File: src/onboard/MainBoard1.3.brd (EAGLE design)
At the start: 134.6 x 80.5 mm, 73 parts, among them IC1 MIC29310-5.0BT, IC2 ADAFRUIT_BMP280, IC3 A5975D

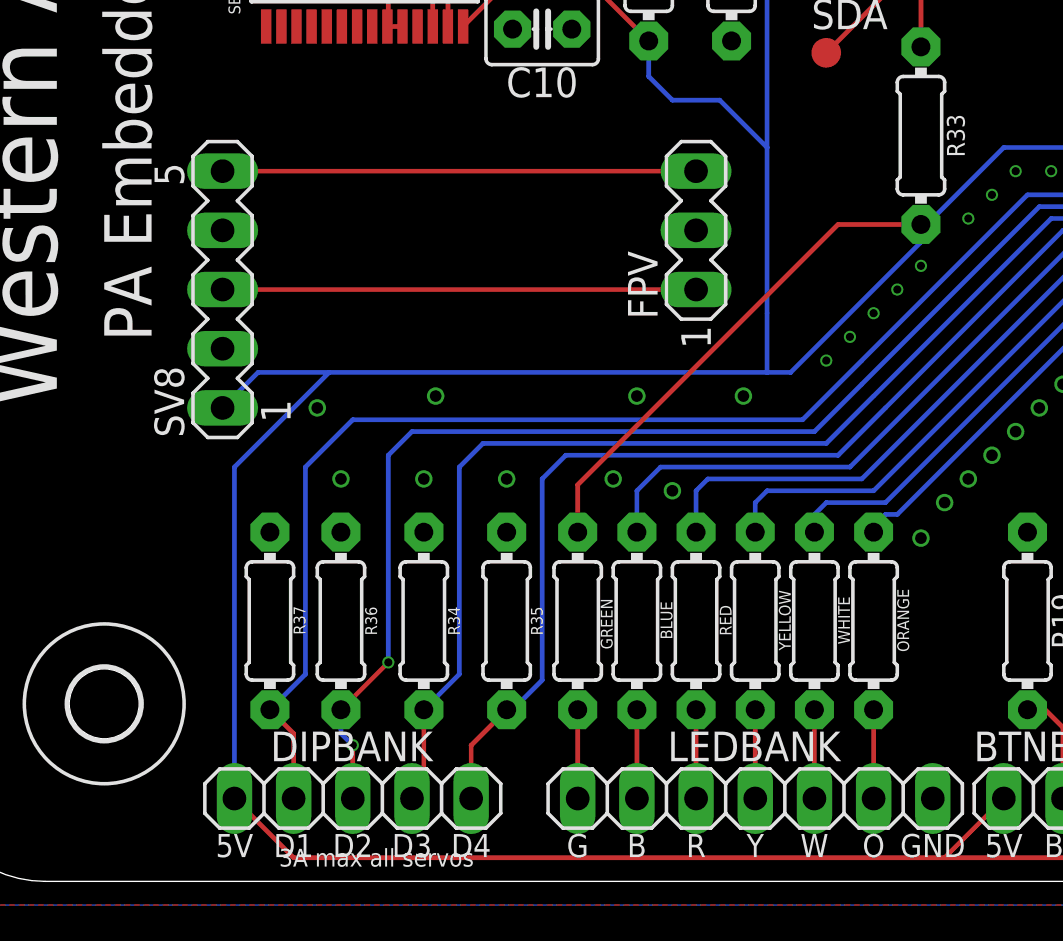
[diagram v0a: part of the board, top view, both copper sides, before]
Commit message: AKK iteration (incomplete)
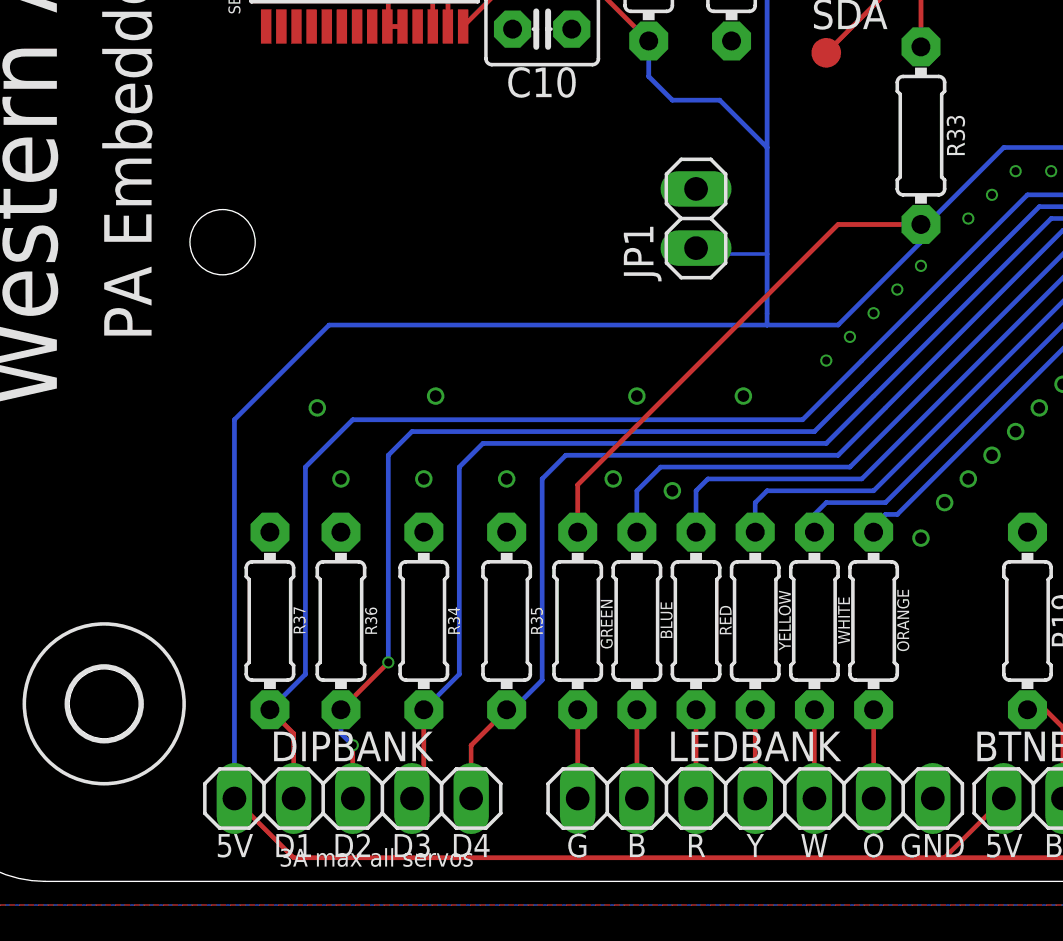
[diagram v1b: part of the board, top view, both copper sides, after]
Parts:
- removed FPV: (no value), con-lstb:MA03-1
- removed SV8: (no value), con-lstb:MA05-1
- added JP1: (no value), pinhead:1X02
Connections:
- removed net VIDEO: FPV.3, SV8.5
- net 5V: now also JP1.1; no longer FPV.1, SV8.1, SV8.3
- net GND: now also JP1.2; no longer FPV.2, SV8.2, SV8.4
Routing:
- net 5V: track 529.3 -> 506.1 mm
- net VIDEO: track 20.3 -> 0.00 mm
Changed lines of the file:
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@@
 <text x="133.096" y="40.259" size="1.778" layer="26" rot="MR90" align="center">Well...it can't get much worse</text>
 <text x="110.236" y="2.159" size="1.778" layer="26" rot="MR180" align="center">It's time to buzz the tower</text>
+<hole x="12.7" y="27.432" drill="2.8"/>
 </plain>
 <attributes>
@@
 <attribute name="VALUE" x="59.69" y="44.704" size="1.27" layer="27" rot="R90" align="center"/>
 </element>
-<element name="FPV" library="con-lstb" library_urn="urn:adsk.eagle:library:162" package="MA03-1" package3d_urn="urn:adsk.eagle:package:8339/1" value="" x="33.02" y="27.94" smashed="yes" rot="R90">
-<attribute name="MF" value="" x="33.02" y="27.94" size="1.778" layer="27" rot="R90" display="off"/>
-<attribute name="MPN" value="" x="33.02" y="27.94" size="1.778" layer="27" rot="R90" display="off"/>
-<attribute name="NAME" x="31.369" y="24.13" size="1.27" layer="25" ratio="10" rot="R90"/>
-<attribute name="OC_FARNELL" value="unknown" x="33.02" y="27.94" size="1.778" layer="27" rot="R90" display="off"/>
-<attribute name="OC_NEWARK" value="unknown" x="33.02" y="27.94" size="1.778" layer="27" rot="R90" display="off"/>
-<attribute name="POPULARITY" value="48" x="33.02" y="27.94" size="1.778" layer="27" rot="R90" display="off"/>
-<attribute name="VALUE" x="35.941" y="24.13" size="1.27" layer="27" ratio="10" rot="R90"/>
-</element>
-<element name="SV8" library="con-lstb" library_urn="urn:adsk.eagle:library:162" package="MA05-1" package3d_urn="urn:adsk.eagle:package:8332/1" value="" x="12.7" y="25.4" smashed="yes" rot="R90">
-<attribute name="MF" value="" x="12.7" y="25.4" size="1.778" layer="27" rot="R90" display="off"/>
-<attribute name="MPN" value="" x="12.7" y="25.4" size="1.778" layer="27" rot="R90" display="off"/>
-<attribute name="NAME" x="11.049" y="19.05" size="1.27" layer="25" ratio="10" rot="R90"/>
-<attribute name="OC_FARNELL" value="unknown" x="12.7" y="25.4" size="1.778" layer="27" rot="R90" display="off"/>
-<attribute name="OC_NEWARK" value="unknown" x="12.7" y="25.4" size="1.778" layer="27" rot="R90" display="off"/>
-<attribute name="POPULARITY" value="29" x="12.7" y="25.4" size="1.778" layer="27" rot="R90" display="off"/>
-<attribute name="VALUE" x="15.621" y="22.86" size="1.27" layer="27" ratio="10" rot="R90"/>
+<element name="JP1" library="pinhead" library_urn="urn:adsk.eagle:library:325" package="1X02" package3d_urn="urn:adsk.eagle:package:22435/2" value="" x="33.02" y="28.448" smashed="yes" rot="R90">
+<attribute name="NAME" x="31.1912" y="25.8318" size="1.27" layer="25" ratio="10" rot="R90"/>
+<attribute name="POPULARITY" value="98" x="33.02" y="28.448" size="1.778" layer="27" rot="R90" display="off"/>
+<attribute name="VALUE" x="36.195" y="25.908" size="1.27" layer="27" rot="R90"/>
 </element>
 </elements>
@@
 <wire x1="32.004" y1="33.528" x2="30.988" y2="34.544" width="0.2032" layer="16"/>
 <wire x1="30.988" y1="34.544" x2="30.988" y2="36.068" width="0.2032" layer="16"/>
-<wire x1="36.068" y1="24.384" x2="36.068" y2="31.496" width="0.2032" layer="16"/>
+<wire x1="36.068" y1="24.384" x2="36.068" y2="26.924" width="0.2032" layer="16"/>
+<wire x1="36.068" y1="26.924" x2="36.068" y2="31.496" width="0.2032" layer="16"/>
 <wire x1="40.132" y1="49.276" x2="36.068" y2="45.212" width="0.2032" layer="16"/>
 <wire x1="36.068" y1="45.212" x2="36.068" y2="31.496" width="0.2032" layer="16"/>
@@
 <wire x1="104.648" y1="59.432" x2="104.648" y2="22.86" width="0.381" layer="1"/>
 <contactref element="IC2" pad="1"/>
-<wire x1="13.208" y1="3.556" x2="13.208" y2="17.78" width="0.2" layer="16"/>
-<wire x1="13.208" y1="17.78" x2="17.272" y2="21.844" width="0.2" layer="16"/>
-<wire x1="17.272" y1="21.844" x2="36.068" y2="21.844" width="0.2" layer="16"/>
-<wire x1="36.068" y1="21.844" x2="37.084" y2="21.844" width="0.2" layer="16"/>
-<wire x1="37.084" y1="21.844" x2="42.672" y2="27.432" width="0.2" layer="16"/>
+<wire x1="13.208" y1="3.556" x2="13.208" y2="19.812" width="0.2" layer="16"/>
+<wire x1="13.208" y1="19.812" x2="17.272" y2="23.876" width="0.2" layer="16"/>
+<wire x1="17.272" y1="23.876" x2="36.068" y2="23.876" width="0.2" layer="16"/>
+<wire x1="36.068" y1="23.876" x2="39.116" y2="23.876" width="0.2" layer="16"/>
+<wire x1="39.116" y1="23.876" x2="42.672" y2="27.432" width="0.2" layer="16"/>
 <wire x1="42.672" y1="27.432" x2="42.672" y2="27.94" width="0.2" layer="16"/>
 <wire x1="42.672" y1="27.94" x2="42.672" y2="28.448" width="0.2" layer="16"/>
-<wire x1="36.068" y1="24.384" x2="36.068" y2="21.844" width="0.2" layer="16"/>
+<wire x1="36.068" y1="24.384" x2="36.068" y2="23.876" width="0.2" layer="16"/>
 <wire x1="78.232" y1="5.08" x2="75.184" y2="8.128" width="0.2" layer="1"/>
 <wire x1="75.184" y1="8.128" x2="73.152" y2="8.128" width="0.2" layer="1"/>
@@
 <wire x1="60.452" y1="31.496" x2="46.228" y2="31.496" width="0.2" layer="16"/>
 <wire x1="46.228" y1="31.496" x2="42.672" y2="27.94" width="0.2" layer="16"/>
-<contactref element="SV8" pad="3"/>
-<contactref element="SV8" pad="1"/>
-<contactref element="FPV" pad="1"/>
-<wire x1="17.272" y1="21.844" x2="14.224" y2="21.844" width="0.2" layer="16"/>
-<wire x1="14.224" y1="21.844" x2="12.7" y2="20.32" width="0.2" layer="16"/>
-<wire x1="12.7" y1="25.4" x2="33.02" y2="25.4" width="0.2" layer="1"/>
+<contactref element="JP1" pad="1"/>
+<wire x1="36.068" y1="26.924" x2="33.528" y2="26.924" width="0.1524" layer="16"/>
+<wire x1="33.528" y1="26.924" x2="33.02" y2="27.432" width="0.1524" layer="16"/>
 <wire x1="73.152" y1="8.128" x2="72.927" y2="7.954" width="0" layer="19" extent="1-1"/>
+<wire x1="33.02" y1="27.178" x2="33.02" y2="27.432" width="0" layer="19" extent="16-16"/>
 <wire x1="42.672" y1="28.194" x2="42.672" y2="28.448" width="0" layer="19" extent="16-16"/>
 <wire x1="25.146" y1="36.576" x2="23.021" y2="36.686" width="0" layer="19" extent="1-1"/>
-<wire x1="12.7" y1="25.4" x2="12.7" y2="20.32" width="0" layer="19" extent="1-1"/>
 </signal>
 <signal name="DIP1">
@@
 <contactref element="C1" pad="2"/>
 <contactref element="IC2" pad="3"/>
-<contactref element="SV8" pad="4"/>
-<contactref element="SV8" pad="2"/>
-<contactref element="FPV" pad="2"/>
+<contactref element="JP1" pad="2"/>
 <wire x1="93.218" y1="77.216" x2="97.536" y2="73.66" width="0" layer="19" extent="1-1"/>
 <wire x1="88.138" y1="73.66" x2="93.218" y2="77.216" width="0" layer="19" extent="1-1"/>
@@
 <wire x1="16.764" y1="20.32" x2="17.78" y2="17.272" width="0" layer="19" extent="1-1"/>
 <wire x1="21.844" y1="20.828" x2="21.336" y2="17.272" width="0" layer="19" extent="1-1"/>
-<wire x1="12.7" y1="22.86" x2="16.764" y2="20.32" width="0" layer="19" extent="1-1"/>
-<wire x1="12.7" y1="27.94" x2="12.7" y2="22.86" width="0" layer="19" extent="1-1"/>
 <wire x1="69.596" y1="24.384" x2="69.596" y2="30.48" width="0" layer="19" extent="1-1"/>
 <wire x1="71.12" y1="24.384" x2="69.596" y2="24.384" width="0" layer="19" extent="1-1"/>
@@
 <wire x1="53.34" y1="48.768" x2="52.324" y2="47.752" width="0" layer="19" extent="1-1"/>
 <wire x1="55.88" y1="48.768" x2="53.34" y2="48.768" width="0" layer="19" extent="1-1"/>
-<wire x1="33.02" y1="27.94" x2="30.48" y2="20.828" width="0" layer="19" extent="1-1"/>
 <wire x1="66.548" y1="12.7" x2="72.927" y2="17.954" width="0" layer="19" extent="1-1"/>
 <wire x1="65.024" y1="14.224" x2="66.548" y2="12.7" width="0" layer="19" extent="1-1"/>
 <wire x1="63.5" y1="12.7" x2="65.024" y2="14.224" width="0" layer="19" extent="1-1"/>
 <wire x1="65.024" y1="11.176" x2="66.548" y2="12.7" width="0" layer="19" extent="1-1"/>
-<wire x1="27.686" y1="36.576" x2="33.02" y2="27.94" width="0" layer="19" extent="1-1"/>
+<wire x1="33.02" y1="29.718" x2="30.48" y2="20.828" width="0" layer="19" extent="1-1"/>
+<wire x1="34.544" y1="36.068" x2="33.02" y2="29.718" width="0" layer="19" extent="1-1"/>
+<wire x1="27.686" y1="36.576" x2="34.544" y2="36.068" width="0" layer="19" extent="1-1"/>
 <wire x1="21.071" y1="36.686" x2="27.686" y2="36.576" width="0" layer="19" extent="1-1"/>
-<wire x1="34.544" y1="36.068" x2="27.686" y2="36.576" width="0" layer="19" extent="1-1"/>
 <wire x1="14.571" y1="42.562" x2="21.071" y2="36.686" width="0" layer="19" extent="1-1"/>
 <wire x1="16.764" y1="50.8" x2="14.571" y2="42.562" width="0" layer="19" extent="1-1"/>
@@
 <wire x1="57.912" y1="68.072" x2="62.23" y2="63.754" width="0.1524" layer="16"/>
 </signal>
-<signal name="VIDEO">
-<contactref element="SV8" pad="5"/>
-<contactref element="FPV" pad="3"/>
-<wire x1="12.7" y1="30.48" x2="33.02" y2="30.48" width="0.2" layer="1"/>
-</signal>
 </signals>
